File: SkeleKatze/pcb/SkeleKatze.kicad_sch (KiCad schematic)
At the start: 6 parts, among them SW1 SW_SPDT

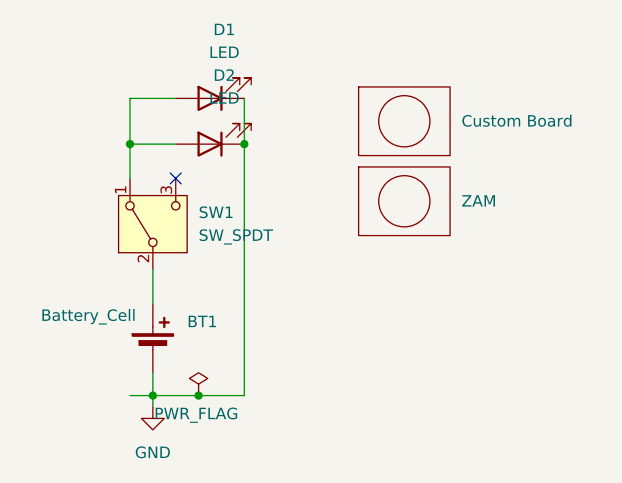
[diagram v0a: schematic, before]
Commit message: Final cut R 1.0
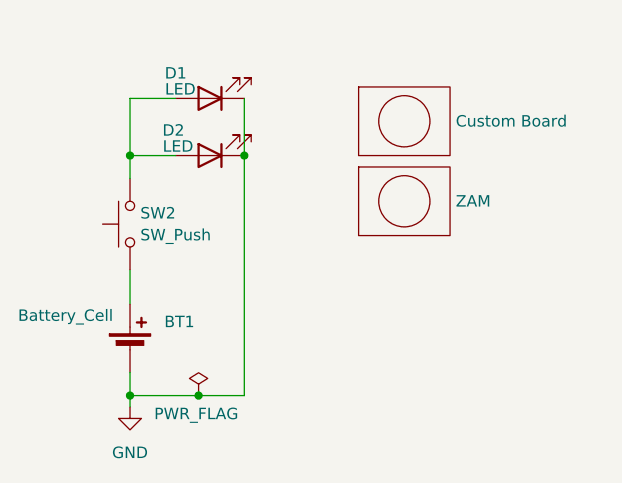
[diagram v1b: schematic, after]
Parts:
- removed SW1: SW_SPDT, Button_Switch_SMD:SW_SPDT_PCM12, symbol Switch:SW_SPDT
- added SW2: SW_Push, ZAM-Parts:SW_PUSH_SPST_ 1208Yd, symbol Switch:SW_Push
- Lg1: footprint SkeleKatze-Lib:SkeleKatze-Combined -> SkeleKatze-Lib:SkeleKatze-Merged; symbol mech:logo -> sjm-mechanical:logo
- Lg2: symbol mech:logo -> sjm-mechanical:logo; now left out of the parts list
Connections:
- net at D1.2 (A), D2.2 (A): now also SW2.2
- net at BT1.1 (+): now also SW2.1
- no-connect marks 1 -> 0
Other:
- moved on the sheet: BT1, D2

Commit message: Creates a Non-Front-Silkscreen version
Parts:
- Lg1: footprint SkeleKatze-Lib:SkeleKatze-Merged -> SkeleKatze-Lib:SkeleKatze-Merged-NFS
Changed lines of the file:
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@@
 			)
 		)
-		(property "Footprint" "SkeleKatze-Lib:SkeleKatze-Merged"
+		(property "Footprint" "SkeleKatze-Lib:SkeleKatze-Merged-NFS"
 			(at 120.65 73.66 0)
 			(hide yes)
